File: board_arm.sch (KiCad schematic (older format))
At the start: 154 parts, among them SW1 SW_Push, SW2 SW_SPDT, U1 STM32F072CBT6, U2 PRTR5V0U2X, U3 MCP1725-3302E_SN

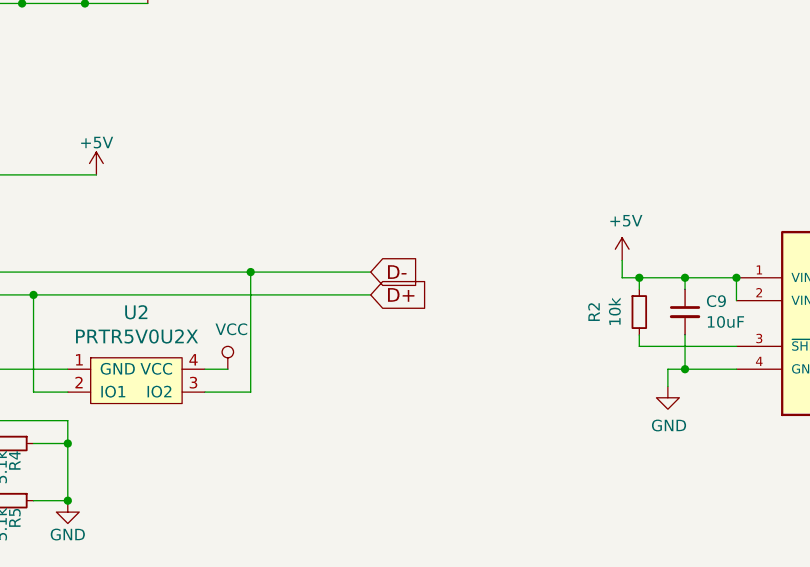
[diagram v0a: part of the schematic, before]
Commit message: Fix MCU wires
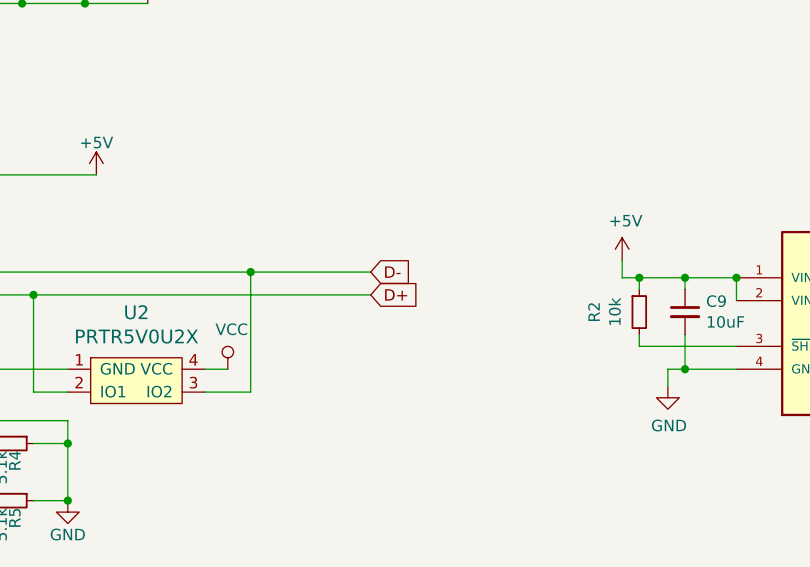
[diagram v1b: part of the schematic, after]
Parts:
- U1: footprint Package_QFP:LQFP-32_7x7mm_P0.8mm -> Package_QFP:LQFP-48_7x7mm_P0.5mm
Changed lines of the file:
@@
 Wire Wire Line
 	1525 5500 1525 5400
-Connection ~ 1525 5400
 Wire Wire Line
 	1525 5200 1525 5100
-Connection ~ 1525 5200
 Connection ~ 1675 5400
-Wire Wire Line
-	1525 5400 1675 5400
 Wire Wire Line
 	1975 5400 1675 5400
 Connection ~ 1675 5200
-Wire Wire Line
-	1675 5200 1975 5200
-Wire Wire Line
-	1675 5200 1525 5200
 Connection ~ 1375 5400
-Wire Wire Line
-	1375 5400 1525 5400
 Wire Wire Line
 	1075 5400 1375 5400
 Connection ~ 1375 5200
-Wire Wire Line
-	1525 5200 1375 5200
 Wire Wire Line
 	1375 5200 1075 5200
@@
 	1    0    0    -1
 $EndComp
-Text GLabel 4050 6575 2    60   Input ~ 0
-D-
-Text GLabel 4050 6675 2    60   Input ~ 0
-D+
 $Comp
 L Type-C:HRO-TYPE-C-31-M-12 USB?
@@
 F 0 "U1" H 3075 1439 50  0000 C CNN
 F 1 "STM32F072CBT6" H 3075 1348 50  0000 C CNN
-F 2 "Package_QFP:LQFP-32_7x7mm_P0.8mm" H 2725 2125 50  0001 R CNN
+F 2 "Package_QFP:LQFP-48_7x7mm_P0.5mm" H 2725 2125 50  0001 R CNN
 F 3 "http://www.st.com/st-web-ui/static/active/en/resource/technical/document/datasheet/DM00105814.pdf" H 3125 3025 50  0001 C CNN
 	1    3125 3025
 	1    0    0    -1
 $EndComp
-Text GLabel 3725 4025 2    50   Input ~ 0
-D+
-Text GLabel 3725 3925 2    50   Input ~ 0
-D-
 Wire Wire Line
 	2575 6675 4050 6675
@@
 Wire Wire Line
 	2800 5400 3075 5400
+Wire Wire Line
+	1375 5400 1525 5400
+Wire Wire Line
+	1525 5400 1675 5400
+Connection ~ 1525 5400
+Wire Wire Line
+	1675 5200 1975 5200
+Wire Wire Line
+	1525 5200 1375 5200
+Wire Wire Line
+	1675 5200 1525 5200
+Connection ~ 1525 5200
+Text GLabel 4050 6575 2    50   Input ~ 0
+D-
+Text GLabel 3725 3925 2    50   Input ~ 0
+D-
+Text GLabel 4050 6675 2    50   Input ~ 0
+D+
+Text GLabel 3725 4025 2    50   Input ~ 0
+D+
 $EndSCHEMATC
